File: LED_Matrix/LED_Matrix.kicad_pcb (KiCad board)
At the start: 2 copper layers, 114.2 x 66.3 mm, 16 parts, among them J1 Conn_01x06_Pin, SW1 SW_SPST, U1 ATtiny85-20P

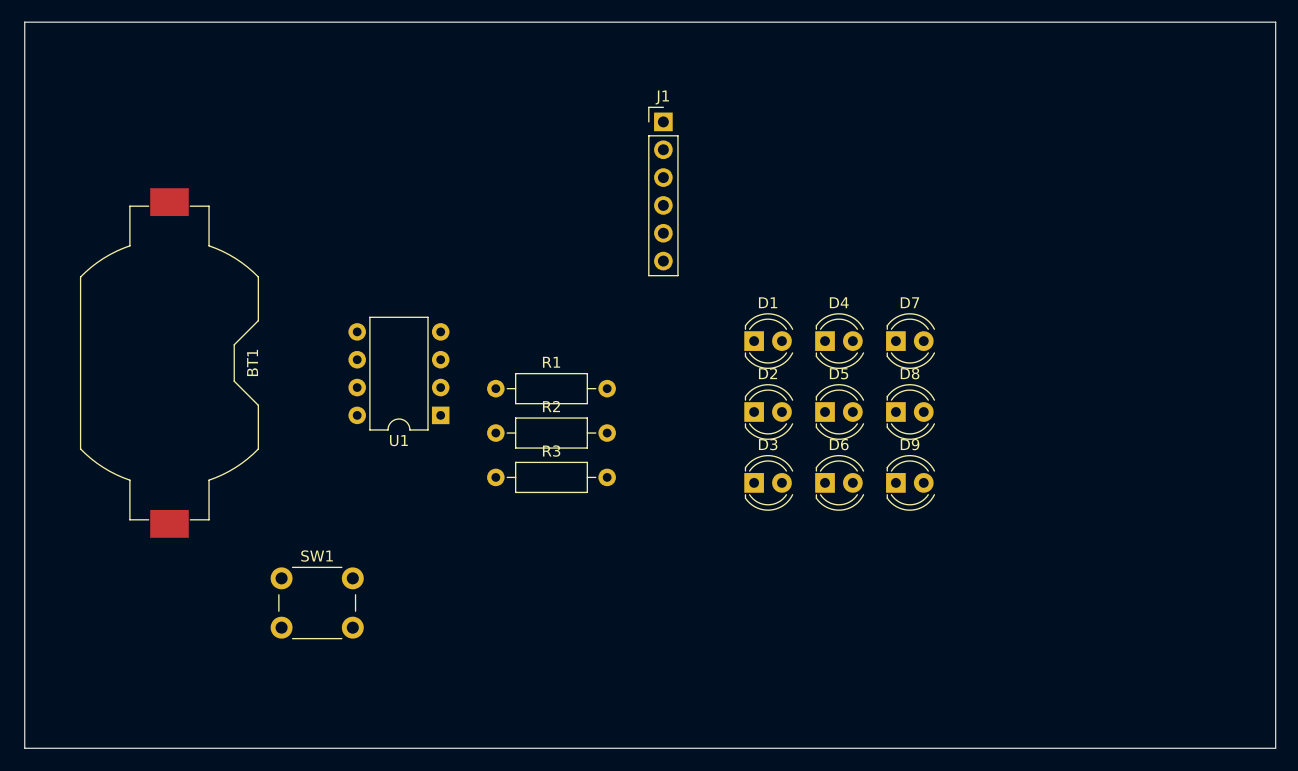
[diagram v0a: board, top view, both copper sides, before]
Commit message: Ass1 Power Supply
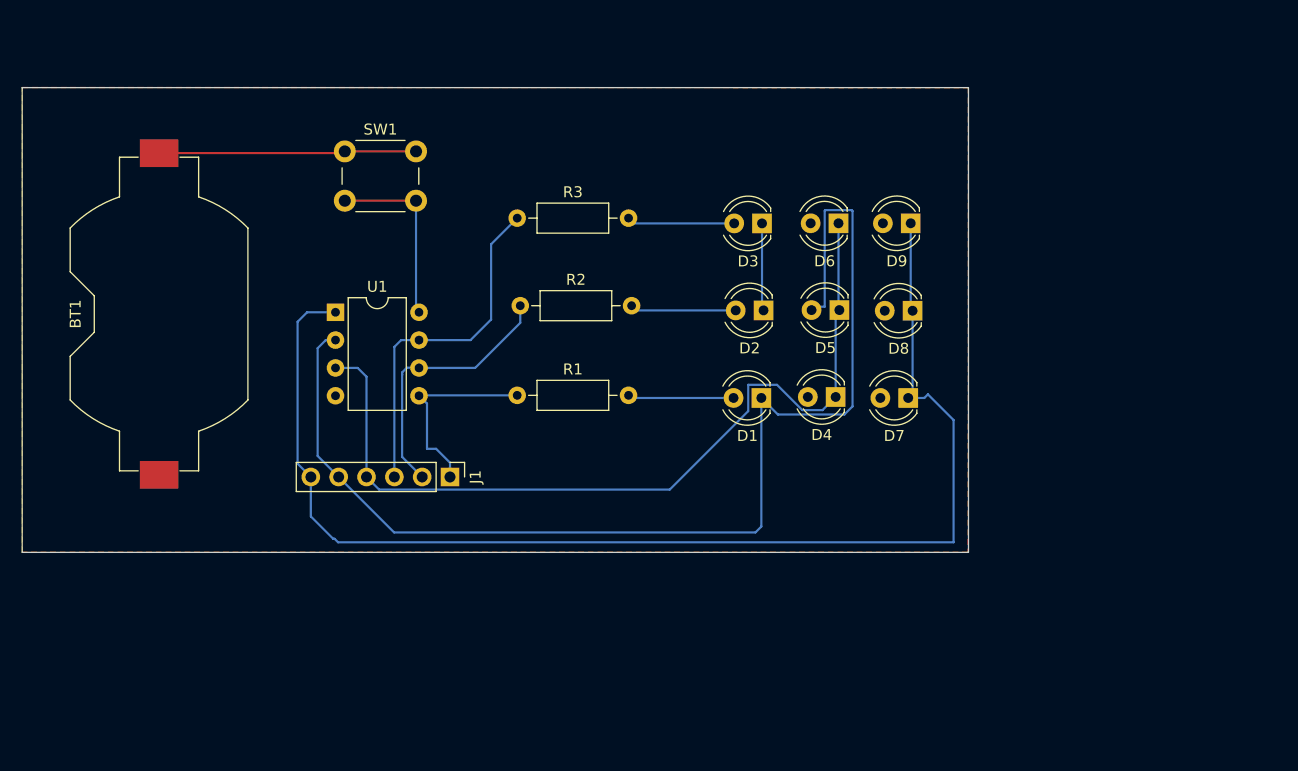
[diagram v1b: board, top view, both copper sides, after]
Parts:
- moved SW1 39.4 mm to (127.7, 64.7)
- moved J1 37.8 mm to (137.3, 94.4), turned to -90 degrees
- moved R3 23.7 mm to (143.4, 70.8)
- moved D9 23.7 mm to (179.3, 71.2), turned to 180 degrees
- moved D6 23.7 mm to (172.8, 71.2), turned to 180 degrees
- moved D3 23.7 mm to (165.8, 71.3), turned to 180 degrees
- moved U1 13.4 mm to (126.9, 79.4), turned to 0 degrees
- moved R2 11.8 mm to (143.7, 78.8)
- moved D5 9.39 mm to (172.8, 79.2), turned to 180 degrees
- moved D8 9.36 mm to (179.5, 79.2), turned to 180 degrees
- moved D2 9.31 mm to (165.9, 79.2), turned to 180 degrees
- moved D7 5.31 mm to (179.1, 87.2), turned to 180 degrees
- moved D1 5.23 mm to (165.7, 87.2), turned to 180 degrees
- moved D4 5.19 mm to (172.5, 87.1), turned to 180 degrees
- moved BT1 4.57 mm to (110.8, 79.5), turned to -90 degrees
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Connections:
- net Net-(BT1-+) renamed /VCC
- net Net-(BT1--) renamed /GND
- J1 pad 4: /C0 -> /C1
- J1 pad 5: /C1 -> /C0
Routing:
- net /C0: track 0.00 -> 114.9 mm
- net /C2: track 0.00 -> 114.3 mm
- net /C1: track 0.00 -> 78.4 mm
- net /R2: track 0.00 -> 32.0 mm
- net /R1: track 0.00 -> 24.6 mm
- net /VCC: track 0.00 -> 23.5 mm
- net /R0: track 0.00 -> 18.1 mm
- net Net-(SW1-B): track 0.00 -> 16.8 mm
- net Net-(D3-A): track 0.00 -> 9.84 mm
- net Net-(D1-A): track 0.00 -> 9.68 mm
- net Net-(D2-A): track 0.00 -> 9.68 mm
- added copper zone on F.Cu, net /GND
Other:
- board size 114.2 x 66.3 mm -> 86.4 x 42.4 mm
